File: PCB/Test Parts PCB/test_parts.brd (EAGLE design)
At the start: 71.1 x 100 mm, 28 parts, among them Y4 20 MHz

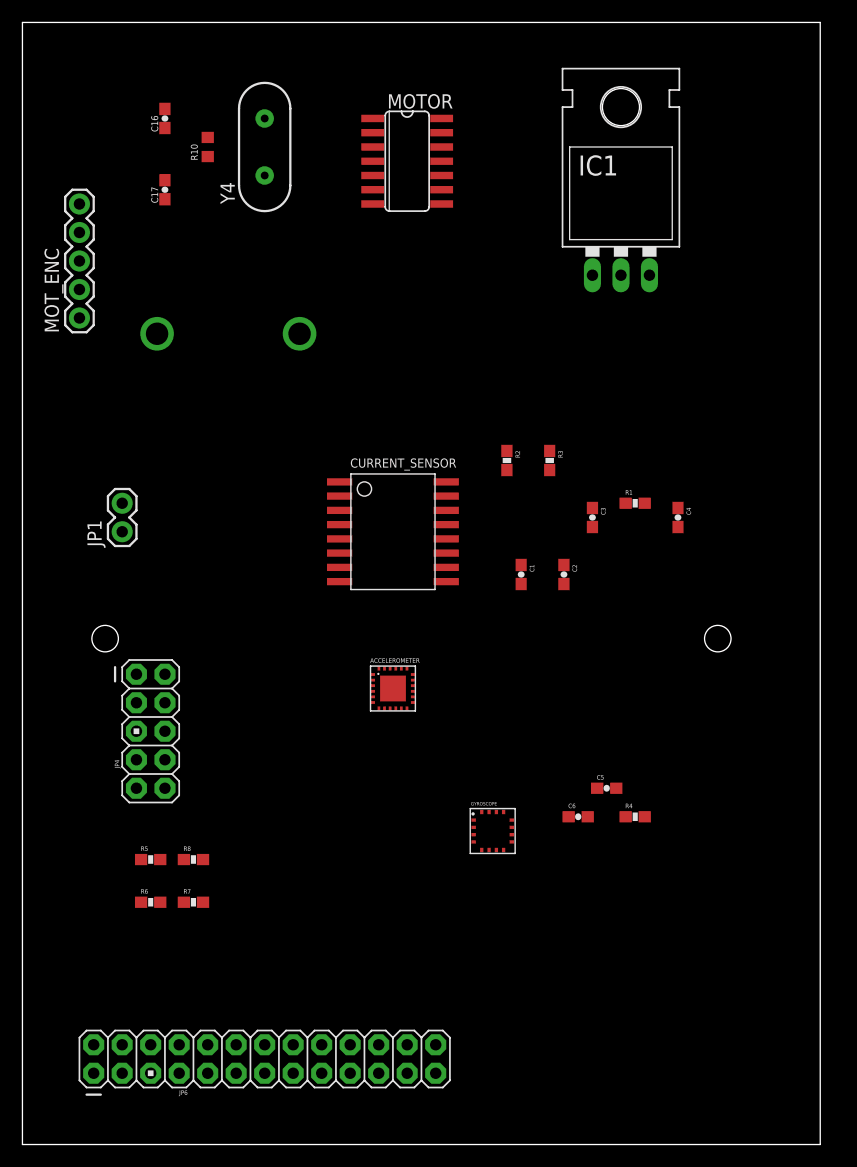
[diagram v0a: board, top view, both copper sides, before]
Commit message: Finished the test PCB
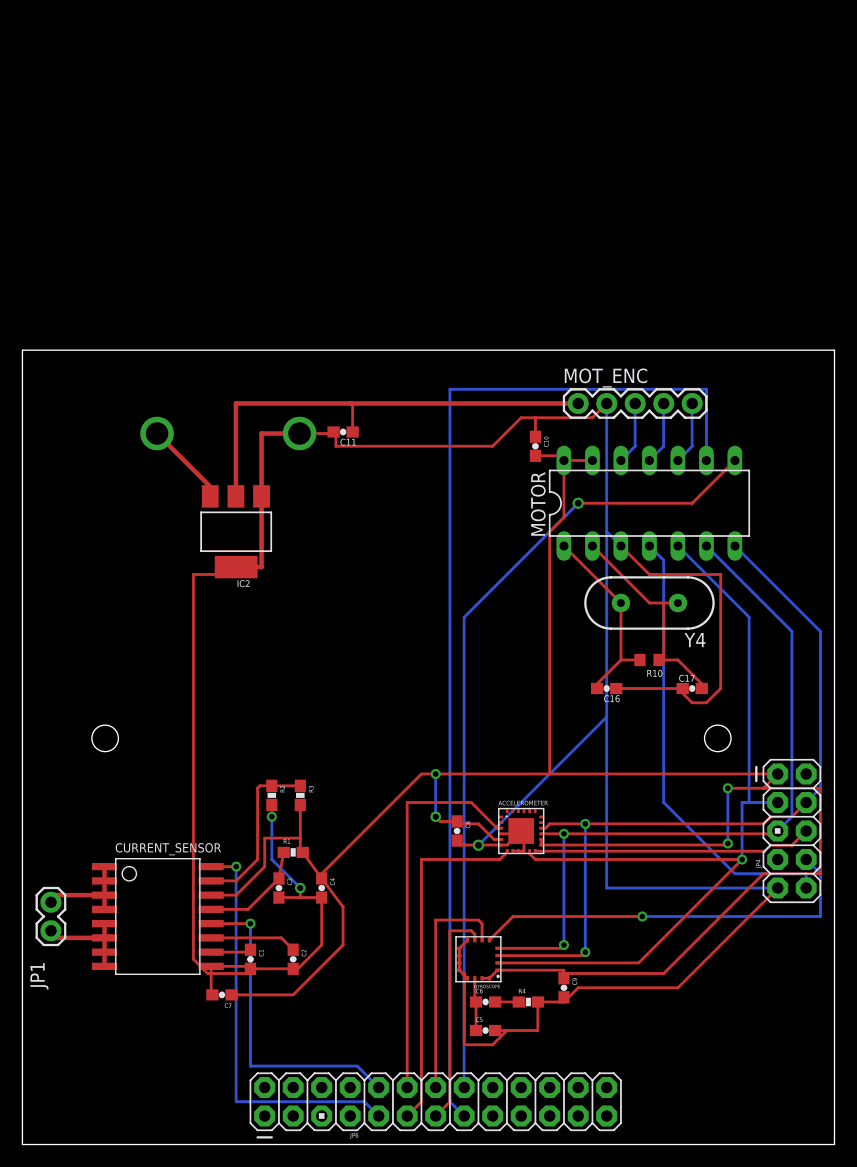
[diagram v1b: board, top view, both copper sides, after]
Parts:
- removed IC1: (no value), SparkFun:TO-220-ALT
- removed R5: 0 Ω, SparkFun:0603-RES
- removed R6, R8: DNI, SparkFun:0603-RES
- removed R7: 1 kΩ, SparkFun:0603-RES
- added C10, C7, C8, C9: 0.1 µF, SparkFun:0603-CAP
- added C11: (no value), nick_nu32_pic32mx795_v1:0603-CAP
- added IC2: REG1117, nick_nu32_pic32mx795_v1:SOT223
- MOTOR: value LS7366R -> LS7366RDIP; device lyndon:SO14 -> lyndon:DIL14
- moved C17 64.7 mm to (59.7, 40.6), turned to 0 degrees
- moved C16 64.3 mm to (52.1, 40.6), turned to 180 degrees
- moved R10 60.3 mm to (55.9, 43.2), turned to 180 degrees
- moved JP4 57.8 mm to (68.6, 27.9)
- moved Y4 53.2 mm to (55.9, 48.3), turned to 180 degrees
- moved C4 45.8 mm to (26.7, 22.9)
- moved MOT_ENC 45.1 mm to (49.5, 66.0), turned to 0 degrees
- moved R1 43.6 mm to (24.1, 26.0)
- moved C3 43.3 mm to (22.9, 22.9)
- moved C1 41.9 mm to (20.3, 16.5)
- moved C2 41.9 mm to (24.1, 16.5)
- moved CURRENT_SENSOR 40.2 mm to (12.1, 20.3)
- moved MOTOR 37.4 mm to (55.9, 57.1), turned to 0 degrees
- moved R3 37.2 mm to (24.8, 31.1)
- moved R2 36.5 mm to (22.2, 31.1)
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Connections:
- removed net CS-OTHER: R6.2, R7.1
- removed net N$11: 4XAA.+, IC1.IN
- removed net N$25: JP6.17
- removed net N$30: JP6.18
- removed net N$9: JP4.10, R5.1, R6.1
- new net N$6: 4XAA.+, IC2.3
- net +5V: now also C11.1, IC2.2; no longer IC1.OUT
- net DIO2: now also JP4.10; no longer R5.2, R8.1
- net GND: now also ACCELEROMETER.HEAT, C10.1, C11.2, C7.2, C8.2, C9.2, GYROSCOPE.9, IC2.1, IC2.4; no longer IC1.GND
- net VCC: now also C10.2, C7.1, C8.1, C9.1; no longer R7.2, R8.2
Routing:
- net GND: track 0.00 -> 290.5 mm, vias 0 -> 3
- net VCC: track 0.00 -> 200.7 mm, vias 0 -> 4
- net DFLAG: track 0.00 -> 94.5 mm
- net SPI_CLK: track 0.00 -> 78.7 mm, vias 0 -> 1
- net LFLAG: track 0.00 -> 71.8 mm, vias 0 -> 1
- net SPI_DOUT: track 0.00 -> 70.7 mm, vias 0 -> 2
- net SPI_DIN: track 0.00 -> 66.5 mm, vias 0 -> 2
- net +5V: track 0.00 -> 41.5 mm
- net DIO2: track 0.00 -> 40.0 mm
- net FAULT_EN: track 0.00 -> 36.4 mm, vias 0 -> 1
- net DIO1: track 0.00 -> 36.0 mm, vias 0 -> 1
- net INT_2: track 0.00 -> 34.7 mm
- net INT_1: track 0.00 -> 31.4 mm
- net VIOUT: track 0.00 -> 28.4 mm, vias 0 -> 1
- net SPI_SS: track 0.00 -> 24.9 mm
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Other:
- board size 71.1 x 100 mm -> 72.4 x 70.8 mm
